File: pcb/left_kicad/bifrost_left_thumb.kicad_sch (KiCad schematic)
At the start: 12 parts, among them J1 Conn_01x06, SW1 UNASSIGNED_41, SW2 UNASSIGNED_42, SW3 UNASSIGNED_43

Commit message: Use Old Norse Bifrǫst spelling
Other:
- title: Bifröst -> Bifrǫst
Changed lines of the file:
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@@
 	(paper "A4")
 	(title_block
-		(title "Bifröst")
+		(title "Bifrǫst")
 		(company "Hringbord")
 		(comment 1 "Generated by Smiðr KiCad export")

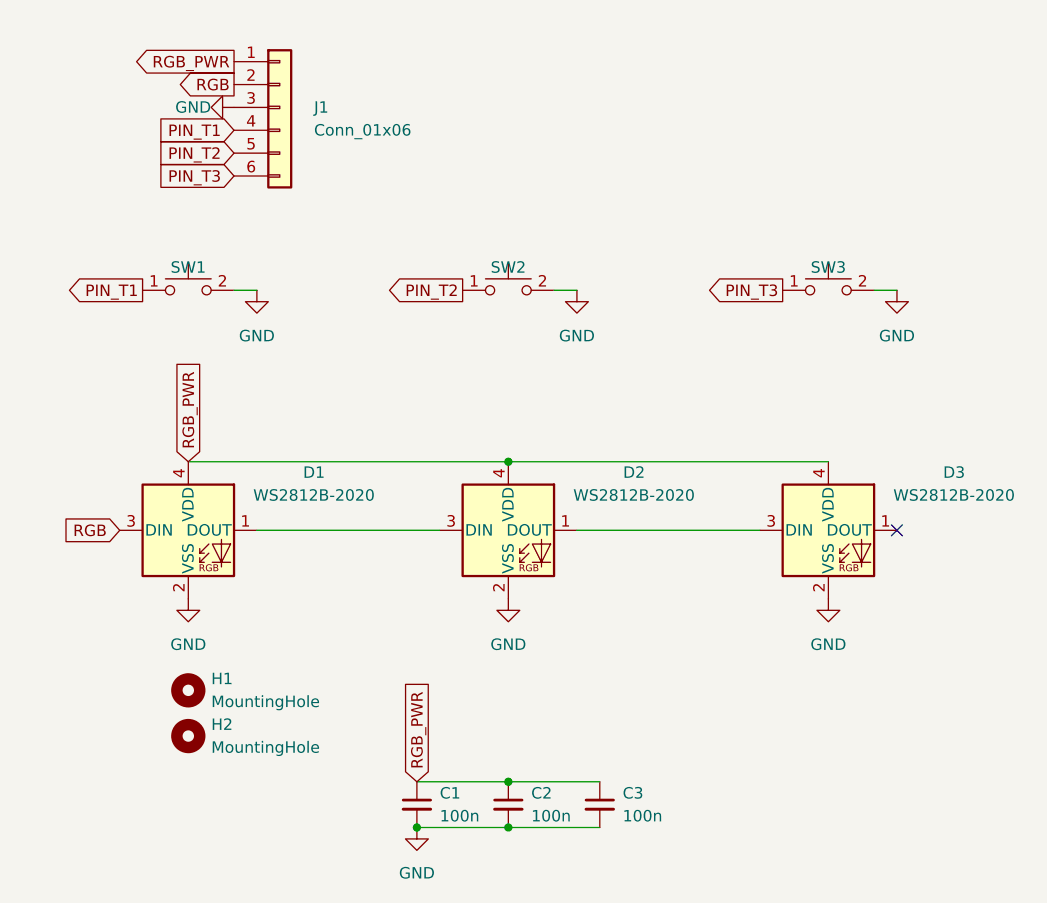
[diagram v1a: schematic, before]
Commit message: Update PCB designs
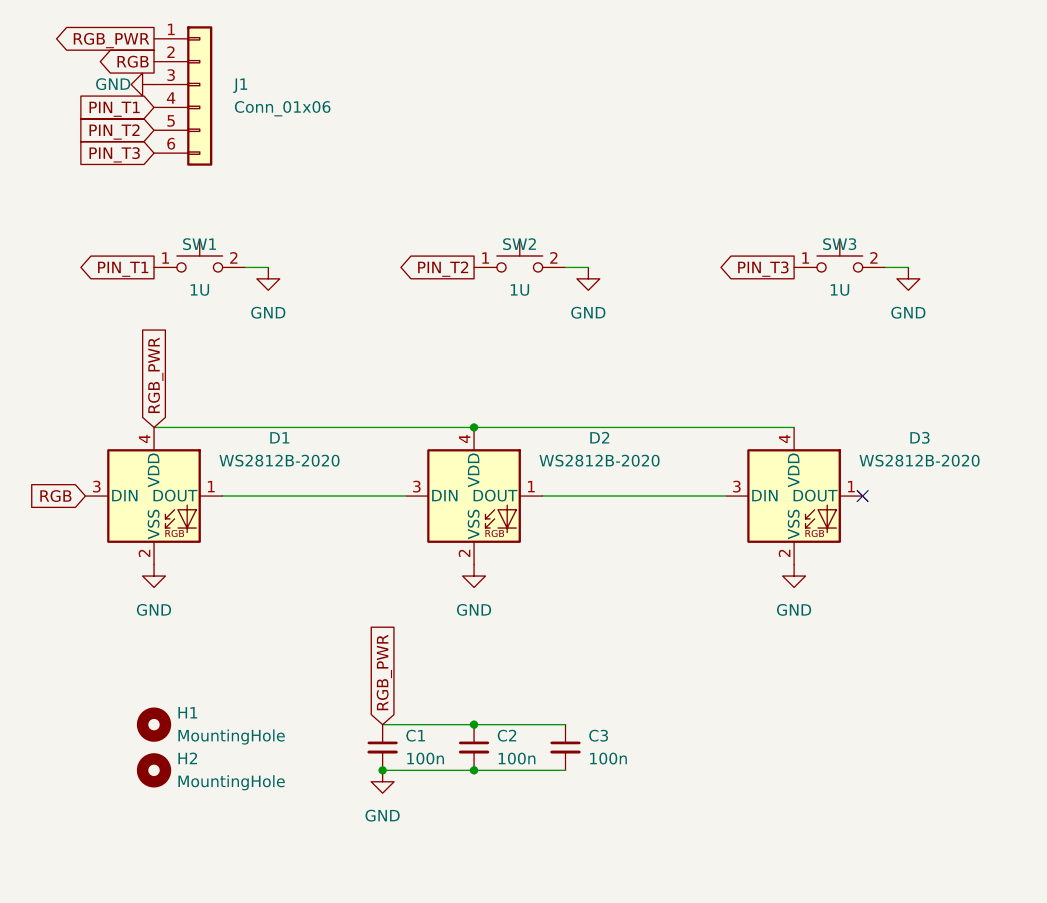
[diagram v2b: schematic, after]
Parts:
- SW1: value UNASSIGNED_41 -> 1U
- SW2: value UNASSIGNED_42 -> 1U
- SW3: value UNASSIGNED_43 -> 1U
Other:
- moved on the sheet: C1, C2, C3, D1, D2, D3, H1, H2, J1, SW1, SW2, SW3
